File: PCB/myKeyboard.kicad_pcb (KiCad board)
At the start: 2 copper layers, 42.5 x 63 mm, 7 parts, among them SW1 SW_Push, SW2 SW_Push, SW3 SW_Push, SW4 SW_Push, U1 XIAO-RP2040-DIP

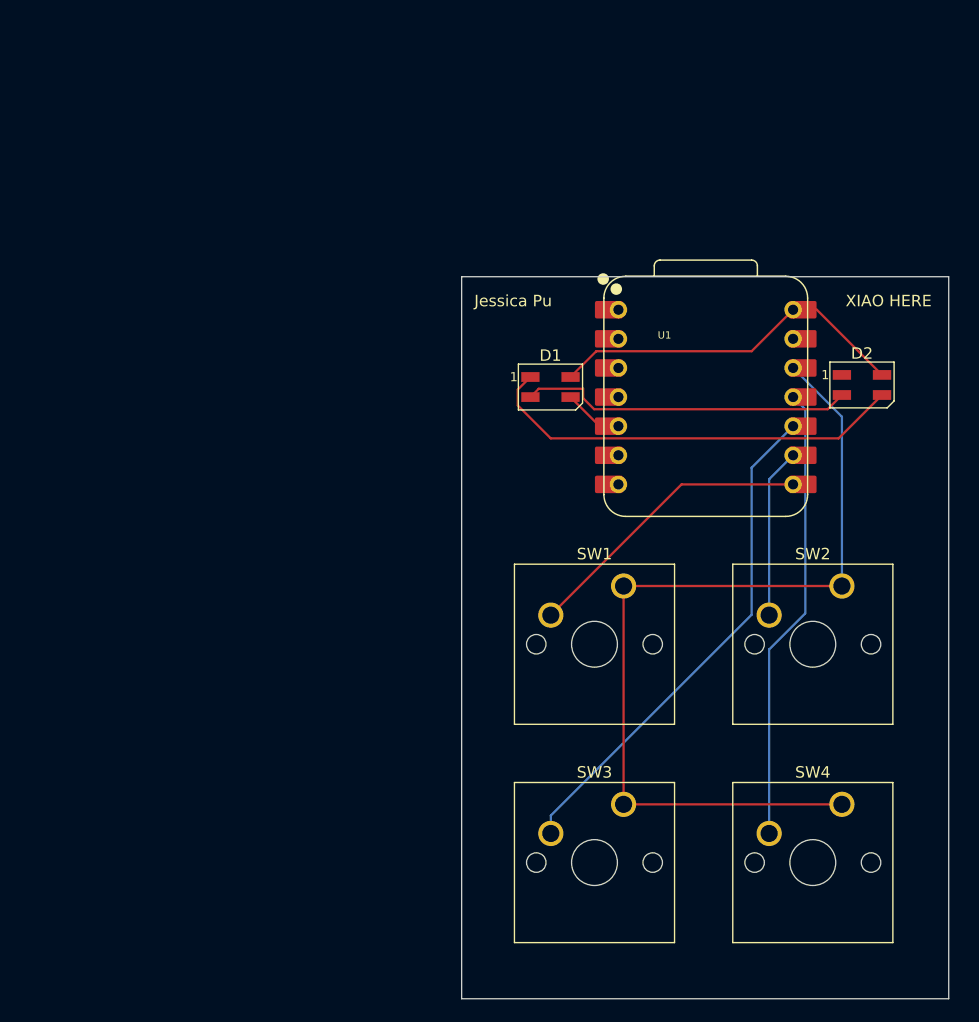
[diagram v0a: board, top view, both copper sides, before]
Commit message: a
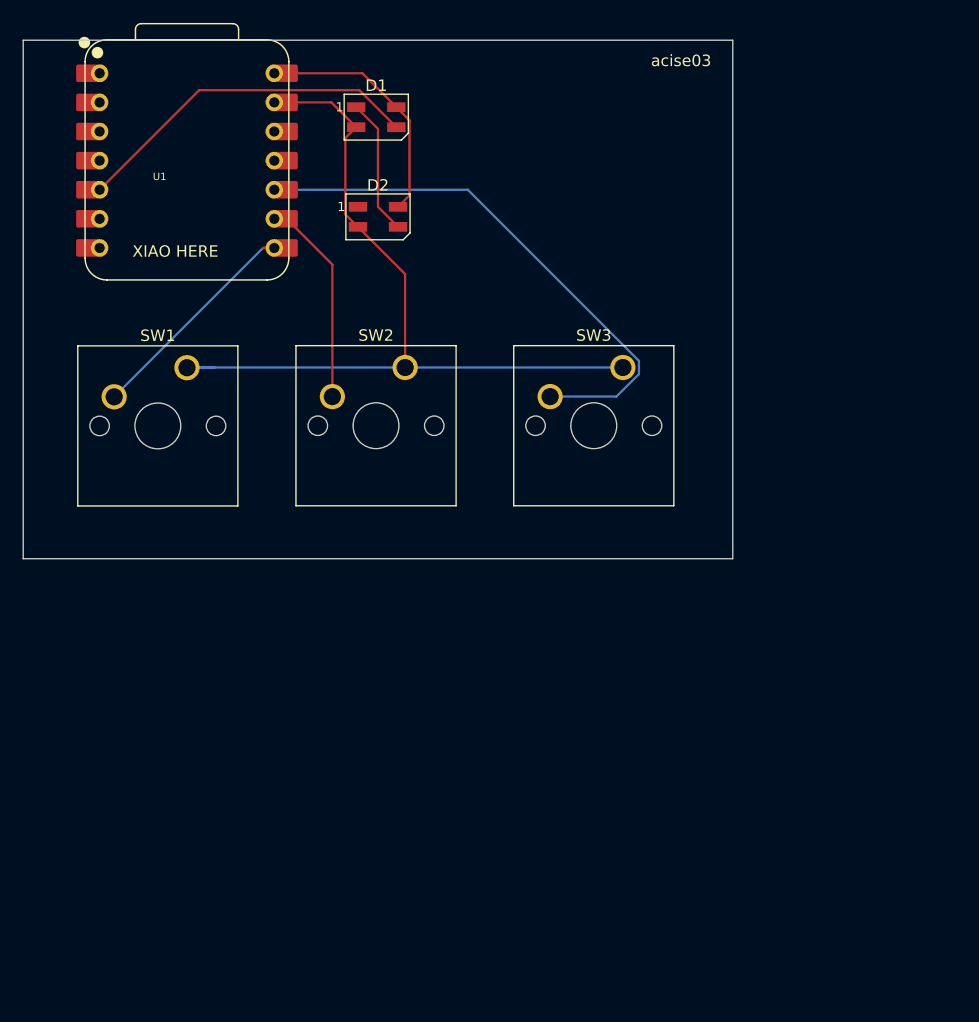
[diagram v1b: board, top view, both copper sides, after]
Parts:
- removed SW4: SW_Push, Button_Switch_Keyboard:SW_Cherry_MX_1.00u_PCB
- moved U1 49.7 mm to (59.5, 53.4)
- moved D2 44.7 mm to (76.2, 58.3)
- moved SW2 42.6 mm to (78.6, 71.4)
- moved SW1 42.6 mm to (59.5, 71.4)
- moved SW3 38.1 mm to (97.6, 71.4)
- moved D1 28.0 mm to (76.0, 49.6)
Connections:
- D1 pad 2: Net-(D1-VSS) -> GND
- D2 pad 2: Net-(D1-VSS) -> GND
- U1 pad 11: Net-(U1-GPIO3/MOSI) -> unconnected-(U1-GPIO3/MOSI-Pad11)
- U1 pad 12: GND -> unconnected-(U1-3V3-Pad12)
- U1 pad 13: unconnected-(U1-GND-Pad13) -> GND
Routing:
- net Net-(U1-GPIO3/MOSI): track 39.8 -> 0.00 mm
- net Net-(D1-VSS): track 29.2 -> 0.00 mm
- net Net-(D1-DIN): track 5.23 -> 30.8 mm
- net Net-(D1-DOUT): track 37.5 -> 12.0 mm
- net +5V: track 32.0 -> 21.5 mm
- net GND: track 77.9 -> 72.0 mm
- net Net-(U1-GPIO1/RX): track 25.9 -> 20.3 mm
- net Net-(U1-GPIO4/MISO): track 44.3 -> 48.8 mm
- net Net-(U1-GPIO2/SCK): track 14.8 -> 18.2 mm
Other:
- board size 42.5 x 63 mm -> 61.9 x 45.2 mm
- board text added: "acise03"
- board text removed: "Jessica Pu"
